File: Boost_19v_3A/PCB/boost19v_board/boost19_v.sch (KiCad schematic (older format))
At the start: 18 parts, among them J1 4P2C, J2 4P2C, U1 circuit

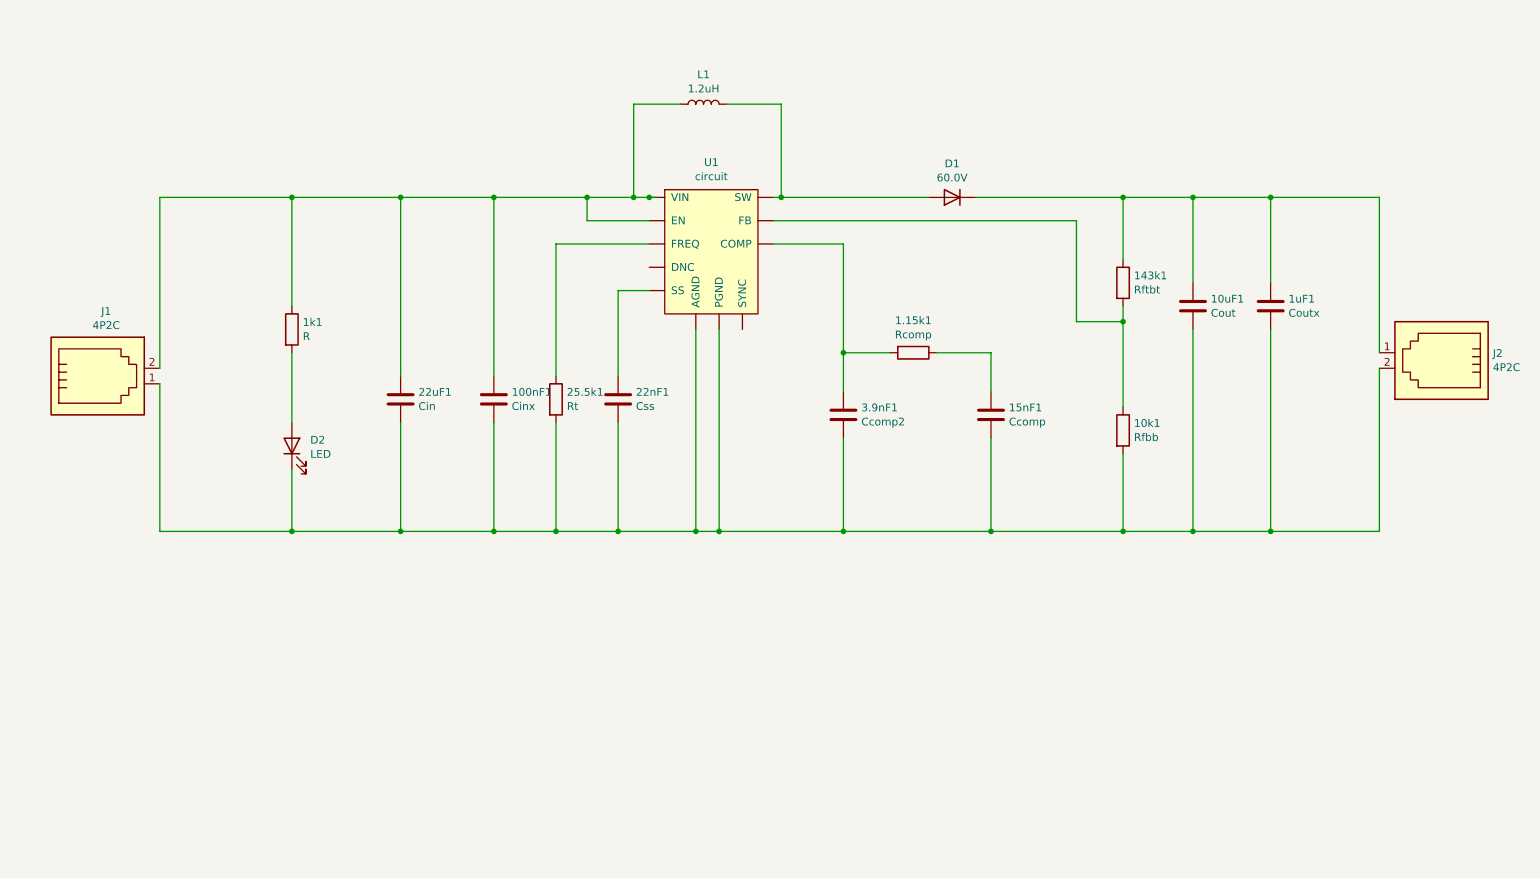
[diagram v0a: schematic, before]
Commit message: boost 19v
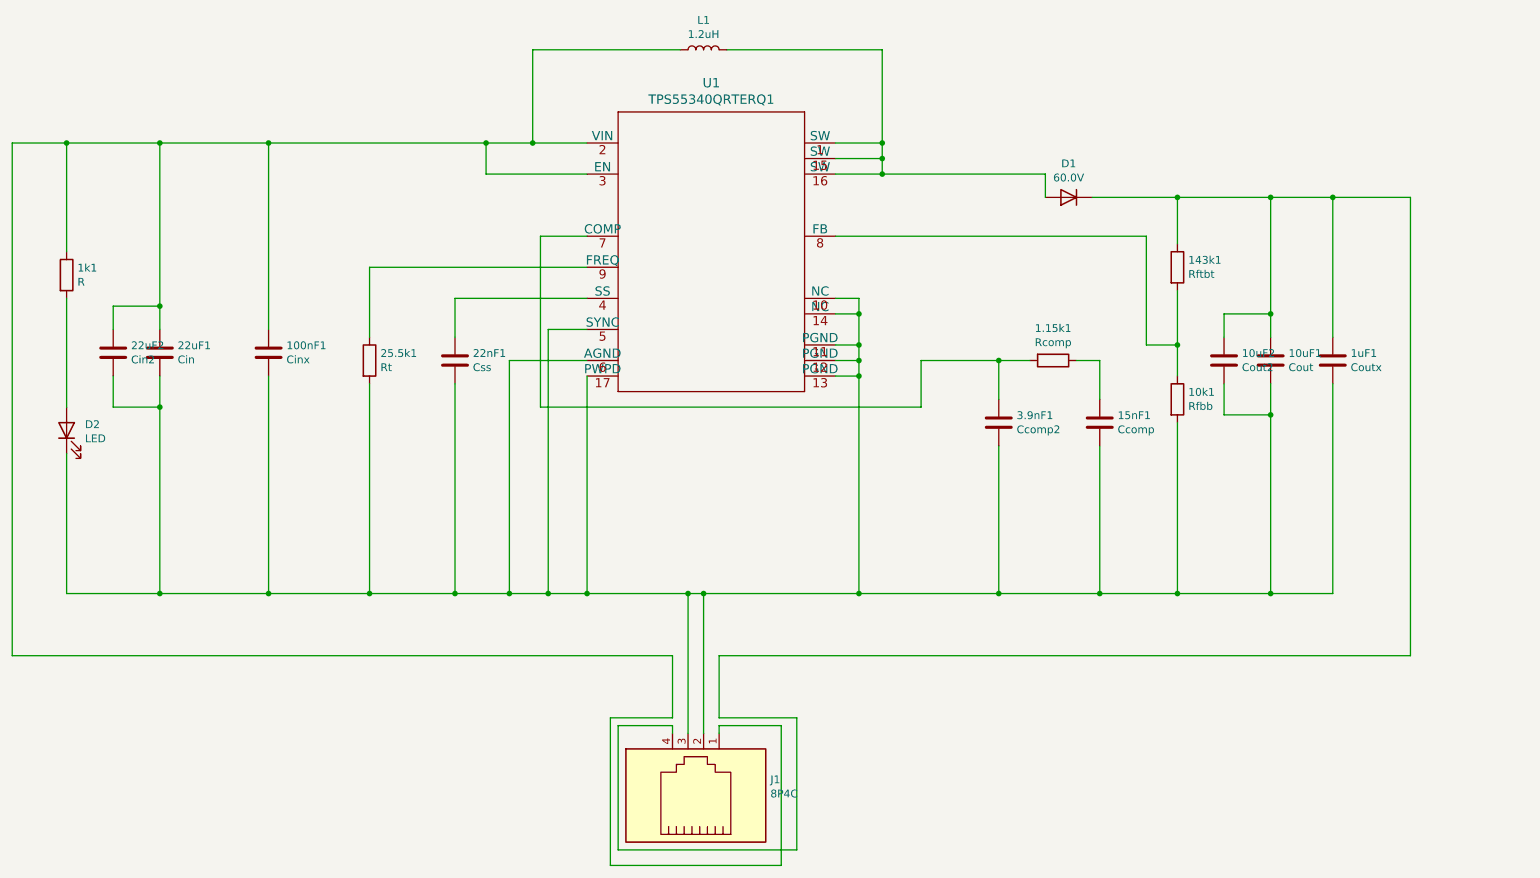
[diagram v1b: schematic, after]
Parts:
- removed J1, J2: 4P2C, 4p2c:43045-0200, symbol connector:4P2C
- removed U1: circuit, IC:TPS55340QRTERQ1, symbol circuit:circuit
- added 10uF2: Cout2, Capacitor_SMD:C_1210_3225Metric_Pad1.33x2.70mm_HandSolder, symbol Device:C
- added 22uF2: Cin2, Capacitor_SMD:C_0805_2012Metric_Pad1.18x1.45mm_HandSolder, symbol Device:C
- added J1: 8P4C, 4x1_connector:436500400, symbol connector:8P4C
- added U1: TPS55340QRTERQ1, IC_update:TPS55340QRTERQ1_002, symbol 2021-01-31_19-46-59:TPS55340QRTERQ1
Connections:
- net at 100nF1.1, 1k1.1, 22uF1.1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: now also 22uF2.1, J1.1, U1.2 (VIN), U1.3 (EN)
- net at D1.2 (A), L1.2: now also U1.1 (SW), U1.15 (SW), U1.16 (SW)
- net at 100nF1.2, 10k1.2, 10uF1.2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: now also 10uF2.2, 22uF2.2, J1.2, J1.3, U1.10 (NC), U1.11 (PGND), U1.12 (PGND), U1.13 (PGND), U1.14 (NC), U1.17 (PWPD), U1.5 (SYNC), U1.6 (AGND)
- net at 25.5k1.1: now also U1.9 (FREQ)
- net at 22nF1.1: now also U1.4 (SS)
- net at 10k1.1, 143k1.2: now also U1.8 (FB)
- net at 1.15k1.2, 3.9nF1.1: now also U1.7 (COMP)
- net at 10uF1.1, 143k1.1, 1uF1.1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: now also 10uF2.1, J1.4
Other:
- moved on the sheet: 1.15k1, 100nF1, 10k1, 10uF1, 143k1, 15nF1, 1k1, 1uF1, 22nF1, 22uF1, 25.5k1, 3.9nF1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
